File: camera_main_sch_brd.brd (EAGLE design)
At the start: 133 x 133 mm, 195 parts, among them CN1 USB C CON, CN2 50 PIN 0.5MM, CN3 31 PIN FPC, CN4 Gb RJ45 + MAG, CN5 USB A, CN6 NO FIT, CN7 uSD, CN8 NO FIT, Q2 SI7489DP, U1 10CL016YF484C6G, U11 USBLC6-2SC6, U12 TPS54233D, U13 FT230X, U14 3.3V BUCK, U15 STUSB4500, U16 Gb PHY, U2 OSD32MP157C-512M-BAA, U3 STM32L431RBT, U4 TLV61046A, U5 AS4C32M16SA, U6 AS4C32M16SA, U7 ACT2861, U8 USBLC6-2SC6, U9 FT232H

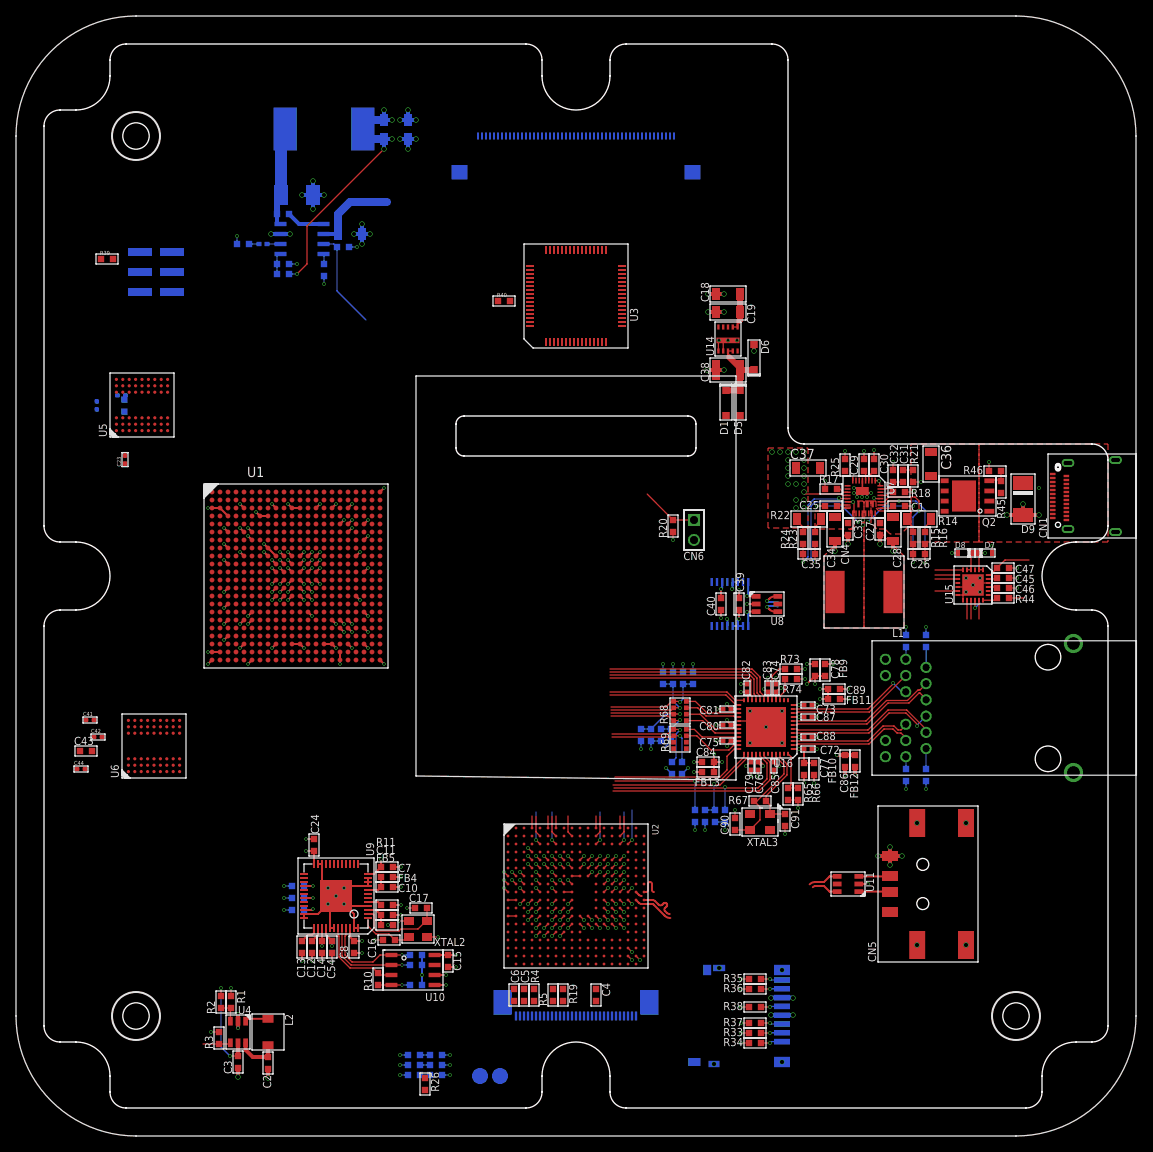
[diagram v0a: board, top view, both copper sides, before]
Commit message: New main PCB started
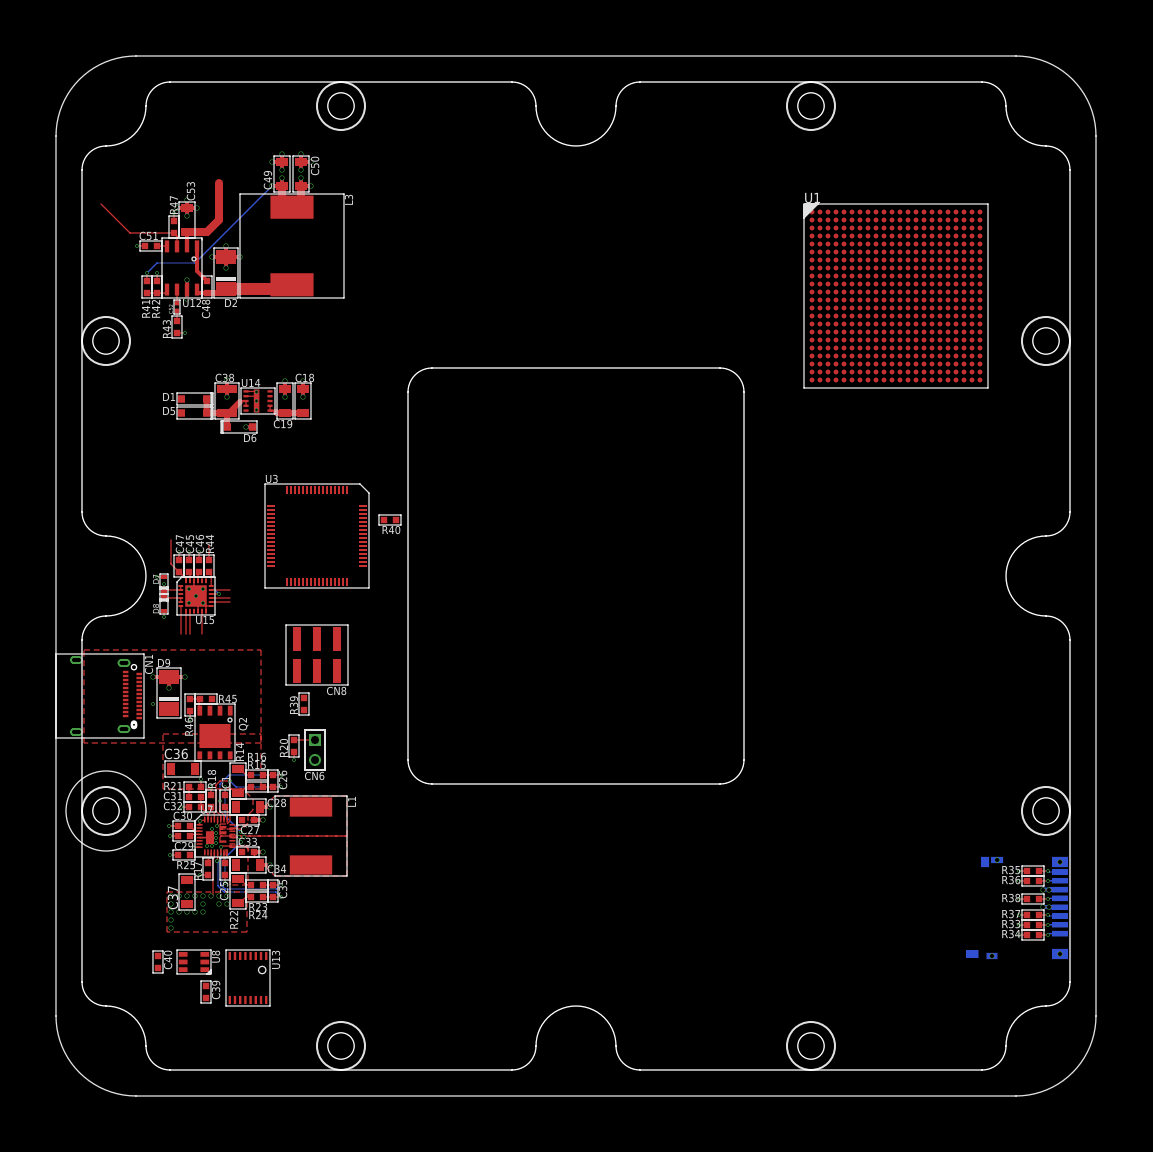
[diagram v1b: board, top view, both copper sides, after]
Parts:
- removed C10, C11, C12, C13, C14, C24, C54, C6, C7, C8: 100nF 16V, CAPACITORS:0603
- removed C15: 100nF 50V, CAPACITORS:0603
- removed C16, C17: 18pF 50V, CAPACITORS:0603
- removed C2, C22, C43, C55: 4.7uF 6.3V, CAPACITORS:0603
- removed C20, C21, C23, C41, C42, C44: 100nF 25V, CAPACITORS:0402@1
- removed C3: 1uF 25V, CAPACITORS:0603
- removed C4, C5: 2.2uF 25V, CAPACITORS:0603
- removed C68, C69, C70, C71: 100nF 100V, CAPACITORS:0603
- removed C72, C73, C74, C75, C76, C79, C80, C81, C82, C83, C85, C87, C88: 100nF 16V, CAPACITORS:0402
- removed C77, C78, C84, C86, C89: 10uF 10V, CAPACITORS:0603
- removed C90, C91: 15pF 50V, CAPACITORS:0603
- removed CN2: 50 PIN 0.5MM, CONNECTORs:FH52E-50S-0.5SH
- removed CN3: 31 PIN FPC, CONNECTORs:3-1734839-1
- removed CN4: Gb RJ45 + MAG, CONNECTORs:0857931020
- removed CN5: USB A, CONNECTORs:629104190121
- removed FB10, FB11, FB12, FB13, FB4, FB5, FB9: 600R, INDUCTORS:0603
- removed L2: 15uH 0.22R, INDUCTORS:DEM3518C
- removed R1: 68k, r_0603:0603
- removed R10: 2.0k, r_0603:0603
- removed R11, R65, R66: 12k, r_0603:0603
- removed R12, R13, R26, R6, R7, R73, R75, R77, R78, R79, R8, R80, R81, R9: 10k, r_0603:0603
- removed R19, R5: 100R, r_0603:0603
- removed R2, R4: 1.0M, r_0603:0603
- removed R27, R28, R29, R30, R31, R32: 10R, r_0603:0603
- removed R3: 100k, r_0603:0603
- removed R67, R71: NO FIT, r_0603:0603
- removed R68, R69: 22R, RESISTORS:1206_ARRAY
- removed R70: 4.7k, r_0603:0603
- removed R72, R74, R76, R82: 1.0k, r_0603:0603
- removed R83, R84, R85: NOT FIT, r_0603:0603
- removed TP1, TP2: 2MM_TEST_POINT, MISC:2MM_TEST_PAD
- removed U10: (no value), ICs:SO8
- removed U11: USBLC6-2SC6, ICs:SOT23-6
- removed U16: Gb PHY, ICs:QFN48_7X7
- removed U2: OSD32MP157C-512M-BAA, Octavo-Systems OSD32MP1:OSD32MP15X-BGA-324
- removed U4: TLV61046A, ICs:SOT23-6
- removed U5, U6: AS4C32M16SA, ICs:FBGA54(8X8)
- removed U9: FT232H, ICs:QFP48_PAD
- removed XTAL2: 12MHz, CRYSTALS:3.2X3.5SMD
- removed XTAL3: 25MHz, CRYSTALS:3.2X2.5SMD
- added MECH4, MECH5, MECH6, MECH7, MECH8: 6mm x 3mm, MISC:MOUNTHOLE_6X3
- moved CN1 126.5 mm to (-59.5, -15.0), turned to 270 degrees
- moved MECH1 116.6 mm to (29.4, 58.8)
- moved D9 109.5 mm to (-50.9, -14.6), turned to 270 degrees
- moved R46 104.8 mm to (-48.2, -16.1), turned to 90 degrees
- moved C47 103.0 mm to (-49.6, 1.25), turned to 270 degrees
- moved R45 102.8 mm to (-46.2, -15.4), turned to 0 degrees
- moved D7 102.7 mm to (-51.5, -1.00), turned to 180 degrees
- moved C45 101.8 mm to (-48.4, 1.25), turned to 270 degrees
- moved C36 101.0 mm to (-49.1, -24.1), turned to 180 degrees
- moved C46 100.5 mm to (-47.1, 1.25), turned to 270 degrees
- moved D8 100.3 mm to (-51.5, -3.50), turned to 0 degrees
- moved R44 99.3 mm to (-45.9, 1.25), turned to 90 degrees
- moved Q2 98.6 mm to (-45.1, -19.5), turned to 270 degrees
- moved R21 97.8 mm to (-47.6, -26.4), turned to 180 degrees
- moved C30 97.3 mm to (-49.0, -31.2), turned to 0 degrees
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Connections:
- removed net 1V2: FB11.2, FB12.2, FB13.2, U1.E17, U1.F6, U1.J10, U1.J11, U1.J12, U1.J13, U1.J14, U1.J8, U1.K14, U1.K9, U1.L14, U1.L9, U1.M14, U1.M9, U1.N9, U1.P10, U1.P11, U1.P12, U1.P13, U1.P9, U1.T13, U1.U16, U1.U17, U1.U6, U1.V17
- removed net 2V5: U1.F18, U1.G6, U1.T6, U1.U18
- removed net 5VUSB: C54.2, C55.2, U2.K9, U9.40
- removed net CMV_LVDS_CLK_IN_N: CN2.P12
- removed net CMV_LVDS_CLK_IN_P: CN2.P13
- removed net CMV_LVDS_CLK_N: CN2.P49
- removed net CMV_LVDS_CLK_P: CN2.P48
- removed net CMV_LVDS_CONT_N: CN2.P15
- removed net CMV_LVDS_CONT_P: CN2.P14
- removed net CMV_LVDS_DATA_11_N: CN2.P25
- removed net CMV_LVDS_DATA_11_P: CN2.P24
- removed net CMV_LVDS_DATA_13_N: CN2.P29
- removed net CMV_LVDS_DATA_13_P: CN2.P28
- removed net CMV_LVDS_DATA_15_N: CN2.P31
- removed net CMV_LVDS_DATA_15_P: CN2.P30
- removed net CMV_LVDS_DATA_17_N: CN2.P34
- removed net CMV_LVDS_DATA_17_P: CN2.P35
- removed net CMV_LVDS_DATA_19_N: CN2.P32
- removed net CMV_LVDS_DATA_19_P: CN2.P33
- removed net CMV_LVDS_DATA_1_N: CN2.P17
- removed net CMV_LVDS_DATA_1_P: CN2.P16
- removed net CMV_LVDS_DATA_21_N: CN2.P38
- removed net CMV_LVDS_DATA_21_P: CN2.P39
- removed net CMV_LVDS_DATA_23_N: CN2.P36
- removed net CMV_LVDS_DATA_23_P: CN2.P37
- removed net CMV_LVDS_DATA_25_N: CN2.P41
- removed net CMV_LVDS_DATA_25_P: CN2.P40
- removed net CMV_LVDS_DATA_27_N: CN2.P43
- removed net CMV_LVDS_DATA_27_P: CN2.P42
- removed net CMV_LVDS_DATA_29_N: CN2.P46
- removed net CMV_LVDS_DATA_29_P: CN2.P47
- removed net CMV_LVDS_DATA_31_N: CN2.P44
- removed net CMV_LVDS_DATA_31_P: CN2.P45
- removed net CMV_LVDS_DATA_3_N: CN2.P20
- removed net CMV_LVDS_DATA_3_P: CN2.P21
- removed net CMV_LVDS_DATA_5_N: CN2.P18
- removed net CMV_LVDS_DATA_5_P: CN2.P19
- removed net CMV_LVDS_DATA_7_N: CN2.P22
- removed net CMV_LVDS_DATA_7_P: CN2.P23
- removed net CMV_LVDS_DATA_9_N: CN2.P26
- removed net CMV_LVDS_DATA_9_P: CN2.P27
- removed net DSP_D_NC: CN3.15
- removed net DSP_IREF: CN3.4, R4.2
- removed net DSP_NRESET: CN3.16
- removed net DSP_SPI_CS: CN3.17
- removed net DSP_SPI_MOSI: R5.2
- removed net DSP_SPI_SCLK: R19.2
- removed net DSP_VCOM: C5.2, CN3.3
- removed net DSP_VDISP_EN: R3.2, U4.4
- removed net ETH_!INT: R71.1, R72.2, U16.38, U2.A4
- removed net ETH_!RST: U16.42
- removed net ETH_CLK125_OUT: R75.1, U16.41, U2.C15
- removed net ETH_MDC: U16.36, U2.B15
- removed net ETH_MDIO: R70.1, U16.37, U2.A15
- removed net ETH_RXC: R69.6, R76.2, U2.C16
- removed net ETH_RXD0: R68.8, R81.1, R85.2, U2.B12
- removed net ETH_RXD1: R68.7, R80.1, R84.2, U2.C12
- removed net ETH_RXD2: R68.6, R79.1, R83.2, U2.B5
- removed net ETH_RXD3: R68.5, R78.1, R82.2, U2.C5
- removed net ETH_RX_CTL: R69.5, R77.1, U2.A12
- removed net ETH_TXC: U16.24, U2.B9
- removed net ETH_TXD0: U16.19, U2.B7
- removed net ETH_TXD1: U16.20, U2.A7
- removed net ETH_TXD2: U16.21, U2.C7
- removed net ETH_TXD3: U16.22, U2.A6
- removed net ETH_TX_CTL: U16.25
- removed net FT232H_3V3: C14.2, C15.2, C24.2, C7.2, C8.2, FB4.1, FB5.1, R12.2, R13.2, R6.2, R7.2, R8.2, R9.2, U10.6, U10.8, U9.12, U9.24, U9.39, U9.46
- removed net FT232H_USB_DM: U2.K18, U9.6
- removed net FT232H_USB_DP: U2.K17, U9.7
- removed net FT_CLK: U9.29
- removed net FT_D0: U9.13
- removed net FT_D1: U9.14
- removed net FT_D2: U9.15
- removed net FT_D3: U9.16
- removed net FT_D4: U9.17
- removed net FT_D5: U9.18
- removed net FT_D6: U9.19
- removed net FT_D7: U9.20
- removed net FT_EE_CLK: R7.1, U10.2, U9.44
- removed net FT_EE_CS: R8.1, U10.1, U9.45
- removed net FT_EE_DI: R10.2, U10.3, U9.43
- removed net FT_NRST: R9.1, U9.34
- removed net FT_OE: U9.30
- removed net FT_PWRSAV1: R13.1, U9.31
- removed net FT_RD: U9.26
- removed net FT_RXF: U9.21
- removed net FT_SIWU1: R12.1, U9.28
- removed net FT_TXE: U9.25
- removed net FT_WR: U9.27
- removed net F_REQ: CN2.P1
- removed net INT1: CN2.P2
- removed net INT2: CN2.P5
- removed net MEM_USB_DM: U11.6, U2.J17
- removed net MEM_USB_DP: U11.4, U2.J18
- removed net MP1_EEPROM_WP: TP1.1, U2.P4
- removed net MP1_PMIC_!PONKEYIN: U2.D3
- removed net MP1_SOFT_!RESET: R26.1, U2.M3
- removed net MP1_USB_VBUS: CN5.1, U11.5
- removed net N$1: R1.2, R2.1, U4.3
- removed net N$100: R73.2, U16.17
- removed net N$101: R74.2, U16.15
- removed net N$13: CN3.11, R5.1
- removed net N$14: CN3.12, R19.1
- removed net N$19: R29.1, R32.2, U2.J6
- removed net N$2: L2.2, U4.1
- removed net N$26: U2.G7, U2.H7, U2.J7, U2.K3, U2.K4, U2.K7, U2.L4, U2.L7, U2.M4, U2.M7
- removed net N$29: R28.1, R31.2, U2.H6
- removed net N$35: U2.J8, U2.J9
- removed net N$36: R27.1, R30.2, U2.G6
- removed net N$37: U2.G10, U2.G9
- removed net N$38: CN5.3, U11.3
- removed net N$39: CN5.2, U11.1
- removed net N$4: C13.2, U9.37
- removed net N$40: U2.K1, U2.K2
- removed net N$41: U2.M1, U2.M2
- removed net N$5: C12.2, U9.38
- removed net N$6: R11.2, U9.5
- removed net N$7: R10.1, R6.1, U10.4
- removed net N$74: CN4.11, U16.2
- removed net N$75: CN4.10, U16.3
- removed net N$76: CN4.4, U16.5
- removed net N$77: CN4.5, U16.6
- removed net N$78: CN4.3, U16.7
- removed net N$79: CN4.2, U16.8
- removed net N$8: C17.2, U9.2, XTAL2.1
- removed net N$80: CN4.8, U16.10
- removed net N$81: CN4.9, U16.11
- removed net N$82: C68.2, CN4.7
- removed net N$83: C69.2, CN4.1
- removed net N$84: C70.2, CN4.6
- removed net N$85: C71.2, CN4.12
- removed net N$86: C74.2, C75.2, C76.2, C78.2, FB9.2, U16.16, U16.34, U16.40
- removed net N$87: C72.2, C73.2, C77.2, FB10.2, U16.1, U16.12
- removed net N$88: C79.2, C80.2, C81.2, C82.2, C83.2, C84.2, FB13.1, U16.18, U16.23, U16.26, U16.30, U16.39
- removed net N$89: C85.2, C86.2, FB12.1, U16.44
- removed net N$9: C16.2, U9.1, XTAL2.3
- removed net N$90: C87.2, C88.2, C89.2, FB11.1, U16.4, U16.9
- removed net N$91: R65.2, R66.2, U16.48
- removed net N$92: C90.2, R67.2, U16.45, XTAL3.3
- removed net N$93: C91.2, R67.1, U16.46, XTAL3.1
- removed net N$94: R68.4, U16.27
- removed net N$95: R68.3, U16.28
- removed net N$96: R68.2, U16.31
- removed net N$97: R68.1, U16.32
- removed net N$98: R69.4, U16.33
- removed net N$99: R69.3, U16.35
- removed net PR_CMV_5V: CN2.P10, CN2.P9
- removed net SDRAM0_!CAS: U6.F7
- removed net SDRAM0_!CS: U6.G9
- removed net SDRAM0_!RAS: U6.F8
- removed net SDRAM0_!WE: U6.F9
- removed net SDRAM0_A0: U6.H7
- removed net SDRAM0_A1: U6.H8
- removed net SDRAM0_A10: U6.H9
- removed net SDRAM0_A11: U6.G2
- removed net SDRAM0_A12: U6.G1
- removed net SDRAM0_A2: U6.J8
- removed net SDRAM0_A3: U6.J7
- removed net SDRAM0_A4: U6.J3
- removed net SDRAM0_A5: U6.J2
- removed net SDRAM0_A6: U6.H3
- removed net SDRAM0_A7: U6.H2
- removed net SDRAM0_A8: U6.H1
- removed net SDRAM0_A9: U6.G3
- removed net SDRAM0_BA0: U6.G7
- removed net SDRAM0_BA1: U6.G8
- removed net SDRAM0_CKE: U6.F3
- removed net SDRAM0_CLK: U6.F2
- removed net SDRAM0_D0: U6.A8
- removed net SDRAM0_D1: U6.B9
- removed net SDRAM0_D10: U6.D1
- removed net SDRAM0_D11: U6.C2
- removed net SDRAM0_D12: U6.C1
- removed net SDRAM0_D13: U6.B2
- removed net SDRAM0_D14: U6.B1
- removed net SDRAM0_D15: U6.A2
- removed net SDRAM0_D2: U6.B8
- removed net SDRAM0_D3: U6.C9
- removed net SDRAM0_D4: U6.C8
- removed net SDRAM0_D5: U6.D9
- removed net SDRAM0_D6: U6.D8
- removed net SDRAM0_D7: U6.E9
- removed net SDRAM0_D8: U6.E1
- removed net SDRAM0_D9: U6.D2
- removed net SDRAM0_LDM: U6.E8
- removed net SDRAM0_UDM: U6.F1
- removed net SDRAM1_!CAS: U5.F7
- removed net SDRAM1_!CS: U5.G9
- removed net SDRAM1_!RAS: U5.F8
- removed net SDRAM1_!WE: U5.F9
- removed net SDRAM1_A0: U5.H7
- removed net SDRAM1_A1: U5.H8
- removed net SDRAM1_A10: U5.H9
- removed net SDRAM1_A11: U5.G2
- removed net SDRAM1_A12: U5.G1
- removed net SDRAM1_A2: U5.J8
- removed net SDRAM1_A3: U5.J7
- removed net SDRAM1_A4: U5.J3
- removed net SDRAM1_A5: U5.J2
- removed net SDRAM1_A6: U5.H3
- removed net SDRAM1_A7: U5.H2
- removed net SDRAM1_A8: U5.H1
- removed net SDRAM1_A9: U5.G3
- removed net SDRAM1_BA0: U5.G7
- removed net SDRAM1_BA1: U5.G8
- removed net SDRAM1_CKE: U5.F3
- removed net SDRAM1_CLK: U5.F2
- removed net SDRAM1_D0: U5.A8
- removed net SDRAM1_D1: U5.B9
- removed net SDRAM1_D10: U5.D1
- removed net SDRAM1_D11: U5.C2
- removed net SDRAM1_D12: U5.C1
- removed net SDRAM1_D13: U5.B2
- removed net SDRAM1_D14: U5.B1
- removed net SDRAM1_D15: U5.A2
- removed net SDRAM1_D2: U5.B8
- removed net SDRAM1_D3: U5.C9
- removed net SDRAM1_D4: U5.C8
- removed net SDRAM1_D5: U5.D9
- removed net SDRAM1_D6: U5.D8
- removed net SDRAM1_D7: U5.E9
- removed net SDRAM1_D8: U5.E1
- removed net SDRAM1_D9: U5.D2
- removed net SDRAM1_LDM: U5.E8
- removed net SDRAM1_UDM: U5.F1
- removed net SPI_EN: CN2.P7
- removed net SPI_MISO: CN2.P6
- removed net SPI_MOSI: CN2.P3
- removed net SPI_SCLK: CN2.P4
- removed net SYS_!RST: CN2.P8
- removed net VDISP: C3.2, C6.2, CN3.2, R2.2, U4.5
- removed net VPHY: C11.2, FB5.2, U9.3
- removed net VPLL: C10.2, FB4.2, U9.8
- net 3V3: no longer C20.2, C21.2, C22.2, C23.2, C41.2, C42.2, C43.2, C44.2, FB10.1, FB9.1, R26.2, R27.2, R28.2, R29.2, R70.2, R71.2, R73.1, R75.2, R77.2, R78.2, R79.2, R80.2, R81.2, U2.H3, U2.J3, U5.A7, U5.A9, U5.B3, U5.C7, U5.D3, U5.E7, U5.J9, U6.A7, U6.A9, U6.B3, U6.C7, U6.D3, U6.E7, U6.J9
- net 3V3_SLP: no longer C2.2, C4.2, CN3.21, L2.1, U4.6
- net 5V: no longer U2.G1, U2.G2, U2.G3, U2.H1, U2.H2, U2.H8, U2.H9, U2.L8, U2.L9, U2.M8, U2.M9
- net GND: no longer C10.1, C11.1, C12.1, C13.1, C14.1, C15.1, C16.1, C17.1, C2.1, C20.1, C21.1, C22.1, C23.1, C24.1, C3.1, C4.1, C41.1, C42.1, C43.1, C44.1, C5.1, C54.1, C55.1, C6.1, C68.1, C69.1, C7.1, C70.1, C71.1, C72.1, C73.1, C74.1, C75.1, C76.1, C77.1, C78.1, C79.1, C8.1, C80.1, C81.1, C82.1, C83.1, C84.1, C85.1, C86.1, C87.1, C88.1, C89.1, C90.1, C91.1, CN2.P11, CN2.P50, CN2.SH1, CN2.SH2, CN3.1, CN3.13, CN3.14, CN3.19, CN3.20, CN3.30, CN3.31, CN4.SH1, CN4.SH2, CN5.4, CN5.SH1, CN5.SH2, CN5.SH3, CN5.SH4, R1.1, R11.1, R3.1, R30.1, R31.1, R32.1, R4.1, R65.1, R66.1, R72.1, R74.1, R76.1, R82.1, R83.1, R84.1, R85.1, TP2.1, U1.A1, U1.A22, U1.AA1, U1.AA17, U1.AA2, U1.AB1, U1.AB17, U1.AB22, U1.AB6, U1.C1, U1.C11, U1.C12, U1.C14, U1.C16, U1.C18, U1.C2, U1.C5, U1.C9, U1.D3, U1.D7, U1.D8, U1.E18, U1.E20, U1.F3, U1.F5, U1.G20, U1.H3, U1.H8, U1.J19, U1.J5, U1.J9, U1.K10, U1.K11, U1.K12, U1.K13, U1.K3, U1.L10, U1.L11, U1.L12, U1.L13, U1.L20, U1.M10, U1.M11, U1.M12, U1.M13, U1.N10, U1.N11, U1.N12, U1.N13, U1.N3, U1.P19, U1.R3, U1.T20, U1.U3, U1.U5, U1.V18, U1.V20, U1.W3, U1.Y11, U1.Y12, U1.Y15, U1.Y16, U1.Y18, U1.Y20, U1.Y5, U1.Y9, U10.5, U11.2, U16.29, U16.PAD, U2.D4, U2.E10, U2.E11, U2.E12, U2.E13, U2.E14, U2.E15, U2.E4, U2.E5, U2.E6, U2.E7, U2.E8, U2.E9, U2.F10, U2.F11, U2.F12, U2.F13, U2.F14, U2.F15, U2.F4, U2.F5, U2.F6, U2.F7, U2.F8, U2.F9, U2.G11, U2.G12, U2.G13, U2.G14, U2.G15, U2.G5, U2.H13, U2.H14, U2.H15, U2.H5, U2.J1, U2.J13, U2.J14, U2.J15, U2.J16, U2.J5, U2.K13, U2.K14, U2.K15, U2.K16, U2.K5, U2.L13, U2.L14, U2.L15, U2.L5, U2.M10, U2.M11, U2.M12, U2.M13, U2.M14, U2.M15, U2.M5, U2.N10, U2.N11, U2.N12, U2.N13, U2.N14, U2.N15, U2.N5, U2.N6, U2.N7, U2.N8, U2.N9, U2.P5, U2.P6, U2.P7, U2.P8, U4.2, U5.A1, U5.A3, U5.B7, U5.C3, U5.D7, U5.E3, U5.J1, U6.A1, U6.A3, U6.B7, U6.C3, U6.D7, U6.E3, U6.J1, U9.10, U9.11, U9.22, U9.23, U9.35, U9.36, U9.4, U9.41, U9.42, U9.47, U9.48, U9.9, U9.PAD, XTAL2.2, XTAL2.4
- net SD_CLK: no longer U2.V17
- net SD_CMD: no longer U2.U18
- net SD_D0: no longer U2.T16
- net SD_D1: no longer U2.U16
- net SD_D2: no longer U2.V16
- net SD_D3: no longer U2.U17
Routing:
- net GND: track 276.8 -> 81.7 mm, vias 280 -> 70
- net N$86: track 31.0 -> 0.00 mm, vias 5 -> 0
- net ETH_CLK125_OUT: track 30.3 -> 0.00 mm, vias 2 -> 0
- net N$88: track 29.6 -> 0.00 mm, vias 7 -> 0
- net ETH_TXD2: track 25.2 -> 0.00 mm, vias 1 -> 0
- net ETH_TXD0: track 25.0 -> 0.00 mm
- net ETH_!INT: track 24.9 -> 0.00 mm, vias 1 -> 0
- net ETH_!RST: track 23.8 -> 0.00 mm
- net FT232H_3V3: track 23.2 -> 0.00 mm, vias 12 -> 0
- net ETH_TXD1: track 23.1 -> 0.00 mm
- net ETH_MDIO: track 22.9 -> 0.00 mm, vias 1 -> 0
- net ETH_TXD3: track 21.8 -> 0.00 mm
- net ETH_MDC: track 20.7 -> 0.00 mm
- net 1V2: track 20.7 -> 0.00 mm, vias 28 -> 0
- net 3V3: track 32.0 -> 11.3 mm, vias 26 -> 10
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- removed copper zone on layer 3, net 1V2
- removed copper zone on layer 3, net 3V3
- removed copper zone on layer 2, net GND
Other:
- board size 133 x 133 mm -> 123.5 x 123.5 mm
